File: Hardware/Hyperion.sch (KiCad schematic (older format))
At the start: 1 part, among them J1 CUBESAT-BUS

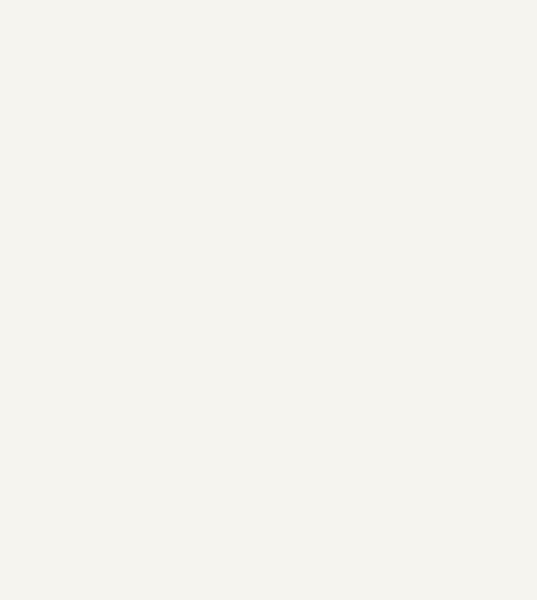
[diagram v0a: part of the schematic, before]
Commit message: Add core components
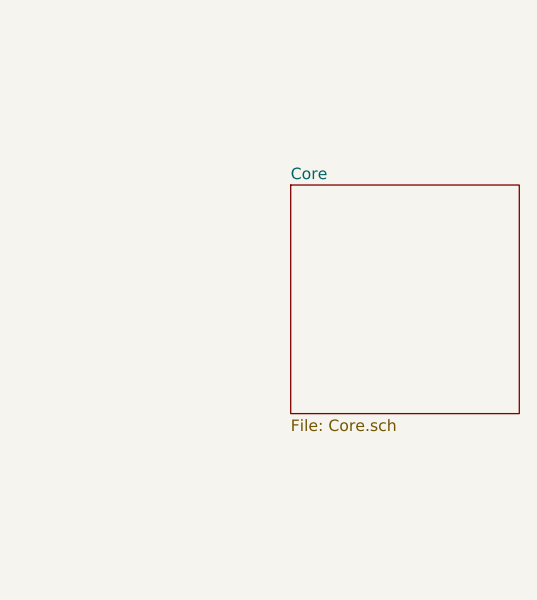
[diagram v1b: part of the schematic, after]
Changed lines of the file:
@@
 LIBS:power
 LIBS:Aerodyne_v2
-EELAYER 24 0
+LIBS:Hyperion-cache
+EELAYER 27 0
 EELAYER END
 $Descr A4 11693 8268
 encoding utf-8
-Sheet 1 1
+Sheet 1 2
 Title ""
-Date ""
+Date "11 oct 2013"
 Rev ""
 Comp ""
@@
 	1    0    0    -1
 $EndComp
+$Sheet
+S 5500 1700 1000 1000
+U 525790DA
+F0 "Core" 50
+F1 "Core.sch" 50
+$EndSheet
 $EndSCHEMATC
